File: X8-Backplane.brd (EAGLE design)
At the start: 122.1 x 122.1 mm, 14 parts, among them U1 LM2678

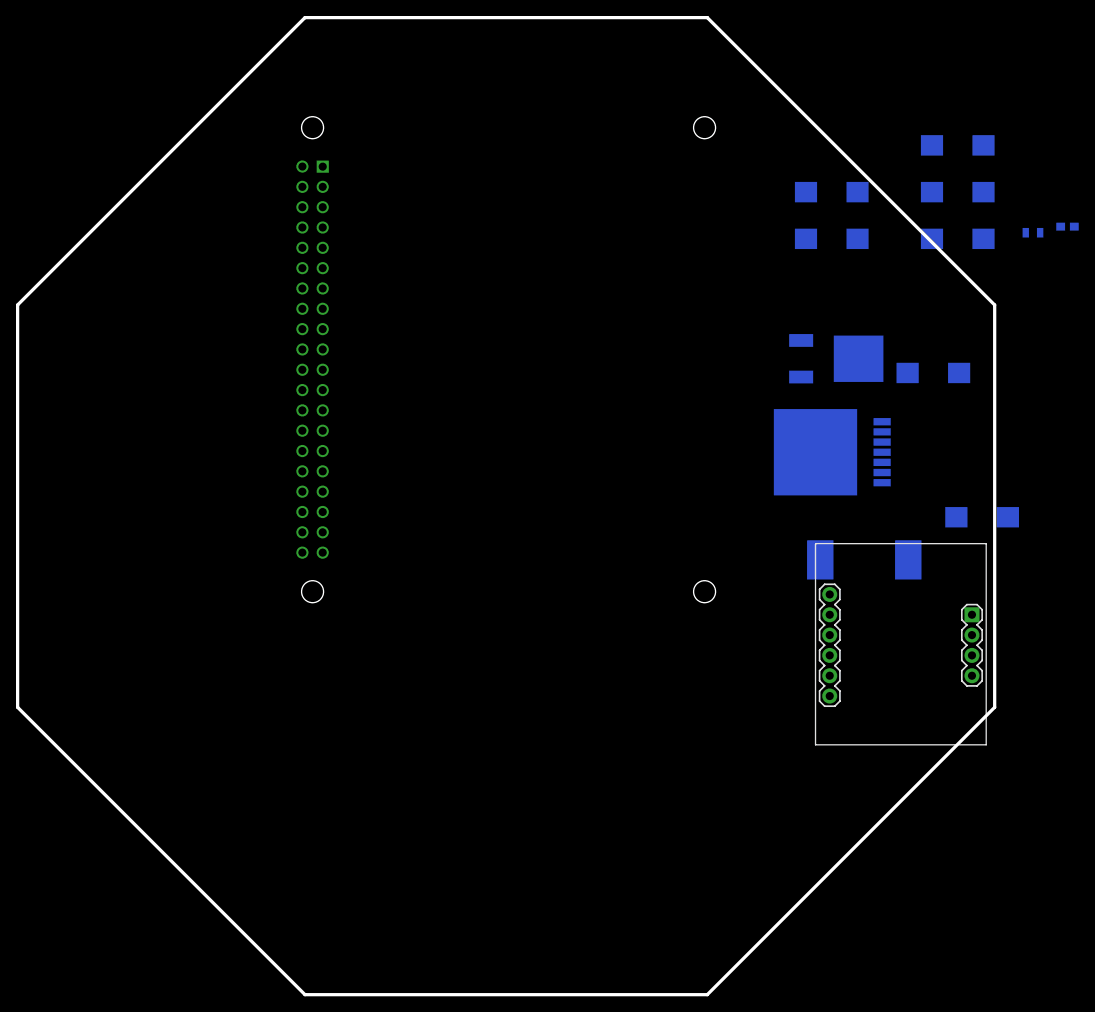
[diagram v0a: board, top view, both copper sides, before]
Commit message: small modification to outline
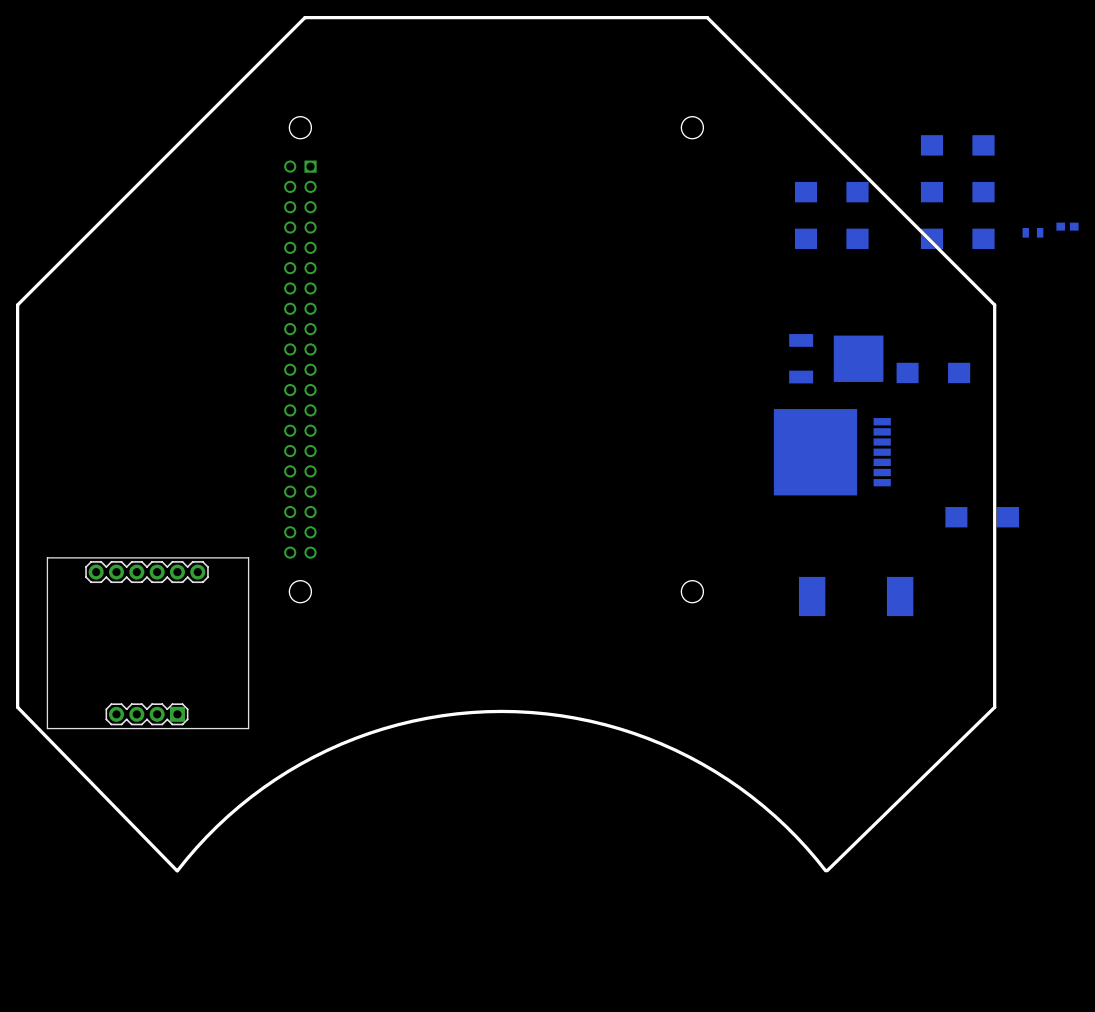
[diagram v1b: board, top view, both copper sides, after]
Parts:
- moved U$3 93.0 mm to (19.8, 21.1), turned to 270 degrees
- moved U$2 4.68 mm to (107.2, 26.9)
- moved PCB1 1.52 mm to (90.2, 89.0)
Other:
- board size 122.1 x 122.1 mm -> 122.1 x 106.6 mm
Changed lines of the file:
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@@
 <circle x="63.43686875" y="38.21558125" radius="73.025" width="0.4064" layer="51"/>
 <wire x1="38.29215" y1="99.28131875" x2="2.371125" y2="63.36029375" width="0.4064" layer="20"/>
-<wire x1="124.50260625" y1="13.0708625" x2="88.581584375" y2="-22.8501625" width="0.4064" layer="20"/>
-<wire x1="2.371125" y1="13.0708625" x2="38.29215" y2="-22.8501625" width="0.4064" layer="20"/>
+<wire x1="124.50260625" y1="13.0708625" x2="103.567584375" y2="-7.3561625" width="0.4064" layer="20"/>
+<wire x1="2.371125" y1="13.0708625" x2="22.29015" y2="-7.3561625" width="0.4064" layer="20"/>
 <wire x1="88.581584375" y1="99.28131875" x2="124.50260625" y2="63.36029375" width="0.4064" layer="20"/>
 <wire x1="88.581584375" y1="99.28131875" x2="38.29215" y2="99.28131875" width="0.4064" layer="20"/>
 <wire x1="124.50260625" y1="63.36029375" x2="124.50260625" y2="13.0708625" width="0.4064" layer="20"/>
-<wire x1="88.581584375" y1="-22.8501625" x2="38.29215" y2="-22.8501625" width="0.4064" layer="20"/>
 <wire x1="2.371125" y1="63.36029375" x2="2.371125" y2="13.0708625" width="0.4064" layer="20"/>
+<wire x1="22.352" y1="-7.366" x2="103.378" y2="-7.366" width="0.4064" layer="20" curve="-104.736525"/>
 </plain>
 <attributes>
@@
 </autorouter>
 <elements>
-<element name="PCB1" library="MicrocontrollerComponents" package="RPI2" value="RPI2" x="91.74" y="89.022" rot="MR270"/>
+<element name="PCB1" library="MicrocontrollerComponents" package="RPI2" value="RPI2" x="90.216" y="89.022" rot="MR270"/>
 <element name="U$1" library="PowerComponents" package="DPAK-3" value="SWITCHMODE_SCHOTTKY" x="104.394" y="56.642" rot="MR0"/>
 <element name="U1" library="PowerComponents" package="LM2678" value="LM2678" x="102.108" y="44.958" rot="MR180"/>
 <element name="C3" library="SparkFun-Capacitors" package="0805" value="0.47uF" x="129.286" y="72.39" rot="MR0"/>
 <element name="C4" library="SparkFun-Passives" package="0603-CAP" value="0.01uF" x="133.604" y="73.152" rot="MR0"/>
-<element name="U$2" library="DiscreteComponents" package="HCMA1305" value="15uH" x="108.204" y="31.496" rot="MR90"/>
+<element name="U$2" library="DiscreteComponents" package="HCMA1305" value="15uH" x="107.188" y="26.924" rot="MR90"/>
 <element name="C6" library="PowerComponents" package="CTAN(7.30_4.30MM)" value="150uF" x="122.936" y="36.83" rot="MR0"/>
 <element name="C9" library="PowerComponents" package="CTAN(7.30_4.30MM)" value="150uF" x="119.888" y="83.312" rot="MR0"/>
@@
 <element name="C13" library="PowerComponents" package="CTAN(7.30_4.30MM)" value="10uF" x="119.888" y="71.628" rot="MR0"/>
 <element name="C2" library="PowerComponents" package="CTAN(7.30_4.30MM)" value="10uF" x="116.84" y="54.864" rot="MR180"/>
-<element name="U$3" library="Other" package="BNO055" value="BNO055_9DOF_BREAKOUT" x="112.776" y="22.098"/>
+<element name="U$3" library="Other" package="BNO055" value="BNO055_9DOF_BREAKOUT" x="19.812" y="21.082" rot="R270"/>
 </elements>
 <signals>
@@
 <contactref element="U$1" pad="P$4"/>
 <wire x1="110.4392" y1="48.768" x2="107.494" y2="56.642" width="0" layer="19" extent="1-1"/>
-<wire x1="113.704" y1="31.496" x2="110.4392" y2="48.768" width="0" layer="19" extent="1-1"/>
+<wire x1="112.688" y1="26.924" x2="110.4392" y2="48.768" width="0" layer="19" extent="1-1"/>
 <wire x1="132.754" y1="73.152" x2="107.494" y2="56.642" width="0" layer="19" extent="1-1"/>
 </signal>
@@
 <wire x1="123.108" y1="83.312" x2="126.156" y2="36.83" width="0" layer="19" extent="1-1"/>
 <wire x1="110.4392" y1="42.418" x2="123.108" y2="83.312" width="0" layer="19" extent="1-1"/>
-<wire x1="102.704" y1="31.496" x2="110.4392" y2="42.418" width="0" layer="19" extent="1-1"/>
+<wire x1="101.688" y1="26.924" x2="110.4392" y2="42.418" width="0" layer="19" extent="1-1"/>
 </signal>
 <signal name="N$4">
